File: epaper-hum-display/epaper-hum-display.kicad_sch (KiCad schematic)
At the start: 31 parts, among them J2 TC2030-SWD, SW1 SW_Push, U1 STM32U575CIT6Q, U10 TCA9416DDF, U9 HDC3022

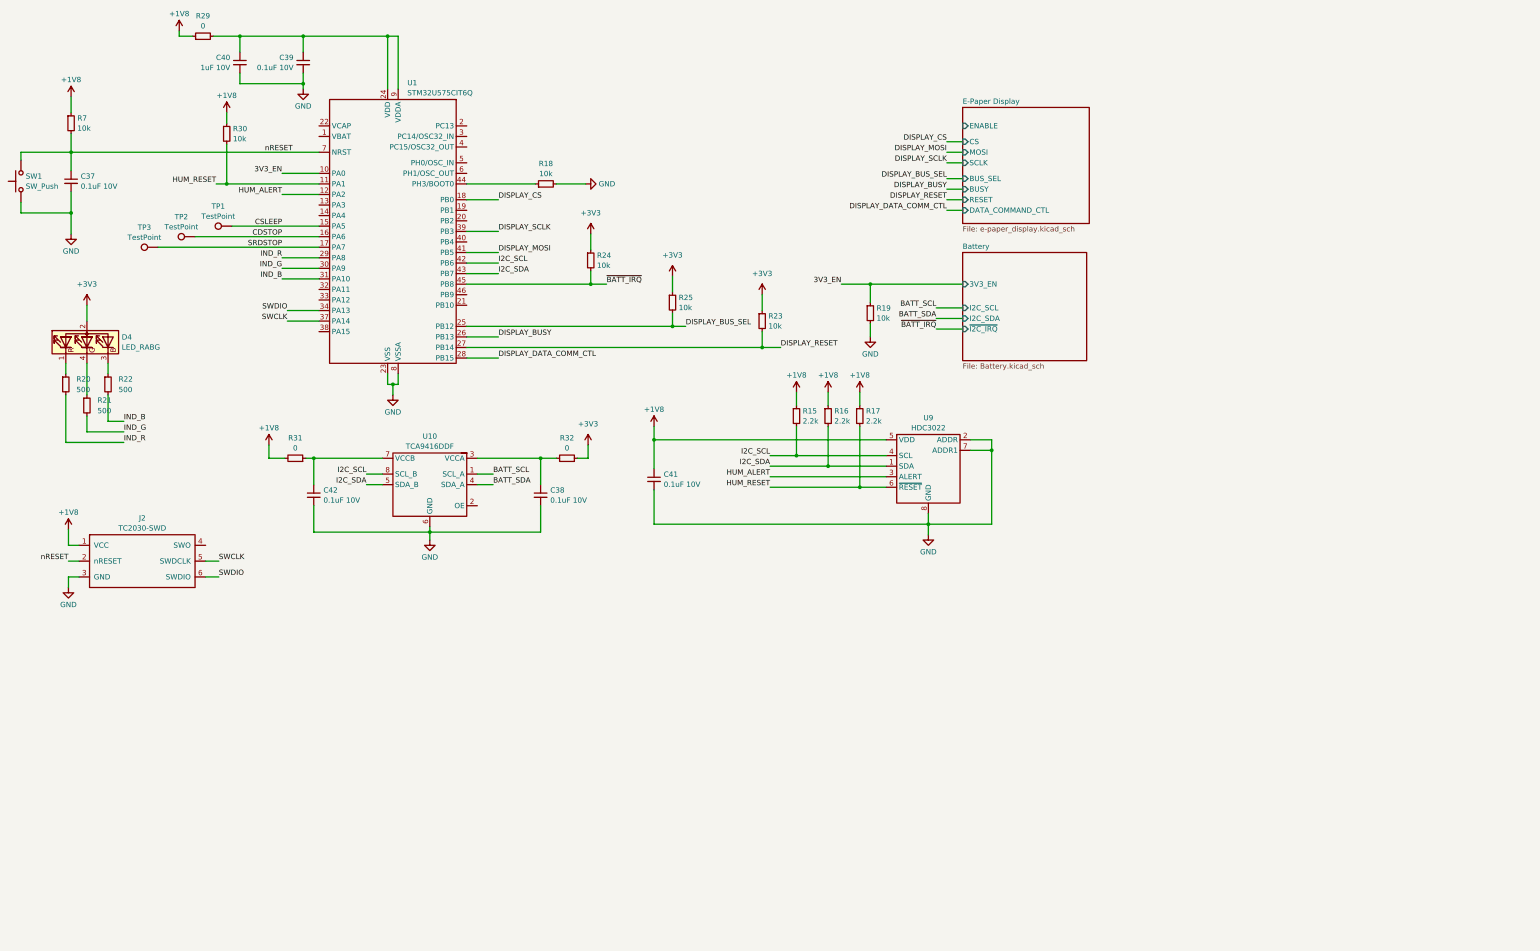
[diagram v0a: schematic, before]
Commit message: WIP
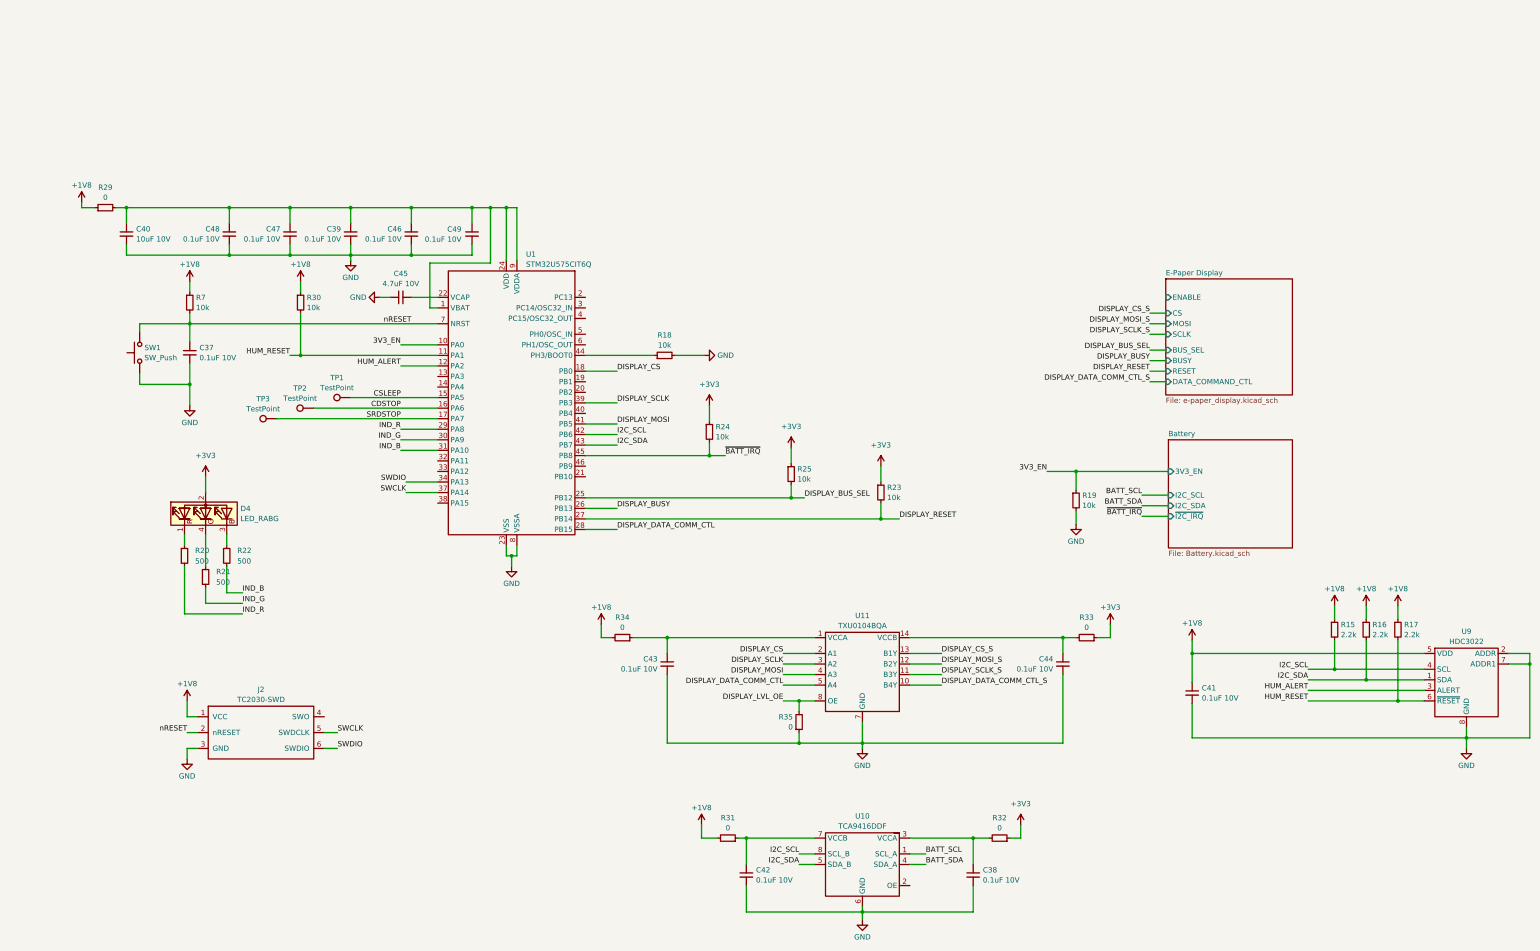
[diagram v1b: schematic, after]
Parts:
- added C43, C44, C46, C47, C48, C49: 0.1uF 10V, symbol Device:C_Small
- added C45: 4.7uF 10V, symbol Device:C_Small
- added R33, R34, R35: 0, symbol Device:R_Small
- added U11: TXU0104BQA, Custom:WQFN-14, symbol Custom:TXU0104BQA
- C40: value 1uF 10V -> 10uF 10V
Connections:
- net +1V8: now also R34.2
- net +3V3: now also R33.1
- net DISPLAY_CS: now also U11.2 (A1)
- net DISPLAY_DATA_COMM_CTL: now also U11.5 (A4)
- net DISPLAY_MOSI: now also U11.4 (A3)
- net DISPLAY_SCLK: now also U11.3 (A2)
- net GND: now also C43.2, C44.2, C45.1, C46.2, C47.2, C48.2, C49.2, R35.1, U11.15 (GND), U11.7 (NC)
- net at C39.1, C40.1, R29.2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: now also U1.1 (VBAT), C46.1, C47.1, C48.1, C49.1
- net at U1.22 (VCAP): now also C45.2
- new net: C43.1, R34.1, U11.1 (VCCA)
- new net: C44.1, R33.2, U11.14 (VCCB)
- new net DISPLAY_CS_S: U11.13 (B1Y)
- new net DISPLAY_DATA_COMM_CTL_S: U11.10 (B4Y)
- new net DISPLAY_LVL_OE: R35.2, U11.8 (OE)
- new net DISPLAY_MOSI_S: U11.12 (B2Y)
- new net DISPLAY_SCLK_S: U11.11 (B3Y)
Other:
- moved on the sheet: C37, C38, C39, C40, C41, C42, D4, J2, R15, R16, R17, R18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
